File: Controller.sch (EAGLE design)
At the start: 5 parts

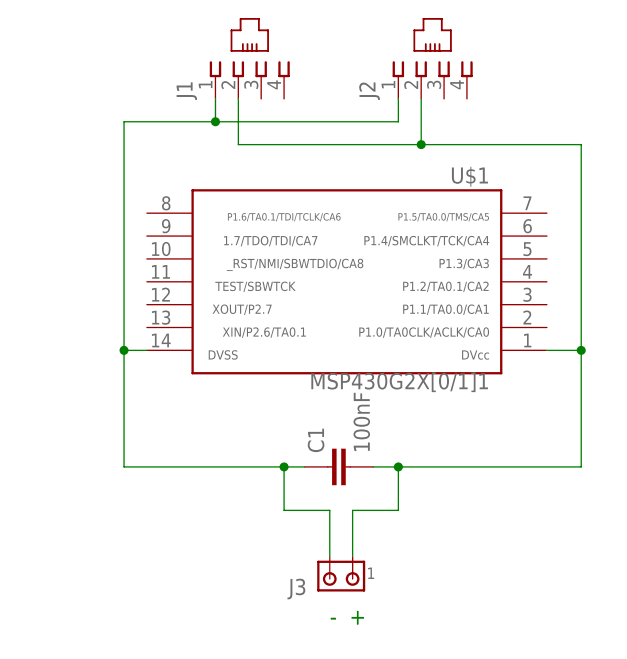
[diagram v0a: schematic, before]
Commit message: final schematics
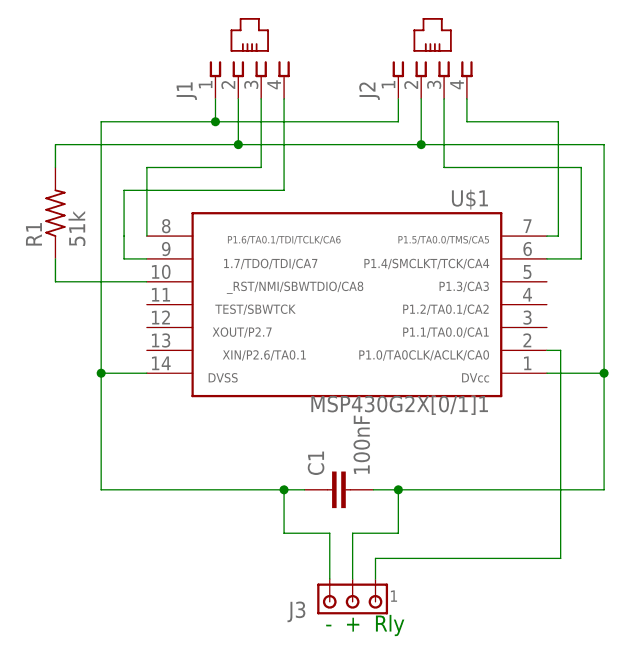
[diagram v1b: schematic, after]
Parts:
- added R1: 51k, resistor:R-US_R0603
- J3: device con-amp:MTA02-156 -> con-amp:MTA03-100
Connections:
- new net N$3: R1.1, U$1.10
- new net N$4: J1.3, U$1.8
- new net N$5: J1.4, U$1.9
- new net N$6: J3.1, U$1.2
- new net N$7: J2.4, U$1.7
- new net N$8: J2.3, U$1.6
- net N$1: now also J3.3; no longer J3.2
- net N$2: now also J3.2, R1.2; no longer J3.1
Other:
- note added: "- + Rly"
- note removed: "- +"
- moved on the sheet: C1, U$1
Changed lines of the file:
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@@
 <part name="J2" library="con-amp" deviceset="555166-3" device=""/>
 <part name="U$1" library="TI_MSP430_v16" deviceset="G2X[0/1]1---N14" device=""/>
-<part name="J3" library="con-amp" deviceset="MTA02-156" device=""/>
+<part name="J3" library="con-amp" deviceset="MTA03-100" device=""/>
 <part name="C1" library="capacitor-wima" deviceset="C" device="2.5/2" value="100nF"/>
+<part name="R1" library="resistor" deviceset="R-US_" device="R0603" value="51k"/>
 </parts>
 <sheets>
 <sheet>
 <plain>
-<text x="43.18" y="12.7" size="1.778" layer="91">-  +</text>
+<text x="42.672" y="11.938" size="1.778" layer="91">-  +  Rly</text>
 </plain>
 <instances>
 <instance part="J1" gate="G$1" x="35.56" y="73.66" rot="R90"/>
 <instance part="J2" gate="G$1" x="55.88" y="73.66" rot="R90"/>
-<instance part="U$1" gate="G$1" x="45.72" y="50.8" rot="R180"/>
-<instance part="J3" gate="G$1" x="45.72" y="17.78" rot="R180"/>
-<instance part="C1" gate="G$1" x="42.926" y="30.226" rot="R90"/>
+<instance part="U$1" gate="G$1" x="45.72" y="48.26" rot="R180"/>
+<instance part="J3" gate="G$1" x="45.72" y="15.24" rot="R180"/>
+<instance part="C1" gate="G$1" x="42.926" y="27.686" rot="R90"/>
+<instance part="R1" gate="G$1" x="12.7" y="58.42" rot="R90"/>
 </instances>
 <busses>
@@
 <segment>
 <pinref part="U$1" gate="G$1" pin="14"/>
-<wire x1="22.86" y1="43.18" x2="20.32" y2="43.18" width="0.1524" layer="91"/>
-<wire x1="20.32" y1="43.18" x2="20.32" y2="30.226" width="0.1524" layer="91"/>
-<wire x1="20.32" y1="30.226" x2="38.1" y2="30.226" width="0.1524" layer="91"/>
-<wire x1="40.386" y1="30.226" x2="38.1" y2="30.226" width="0.1524" layer="91"/>
-<wire x1="38.1" y1="30.226" x2="38.1" y2="25.4" width="0.1524" layer="91"/>
-<pinref part="J3" gate="G$1" pin="2"/>
-<wire x1="38.1" y1="25.4" x2="43.18" y2="25.4" width="0.1524" layer="91"/>
-<wire x1="43.18" y1="25.4" x2="43.18" y2="20.32" width="0.1524" layer="91"/>
-<junction x="38.1" y="30.226"/>
-<wire x1="20.32" y1="43.18" x2="20.32" y2="68.58" width="0.1524" layer="91"/>
+<wire x1="22.86" y1="40.64" x2="17.78" y2="40.64" width="0.1524" layer="91"/>
+<wire x1="17.78" y1="40.64" x2="17.78" y2="27.686" width="0.1524" layer="91"/>
+<wire x1="17.78" y1="27.686" x2="38.1" y2="27.686" width="0.1524" layer="91"/>
+<wire x1="40.386" y1="27.686" x2="38.1" y2="27.686" width="0.1524" layer="91"/>
+<wire x1="38.1" y1="27.686" x2="38.1" y2="22.86" width="0.1524" layer="91"/>
+<pinref part="J3" gate="G$1" pin="3"/>
+<wire x1="38.1" y1="22.86" x2="43.18" y2="22.86" width="0.1524" layer="91"/>
+<wire x1="43.18" y1="22.86" x2="43.18" y2="17.78" width="0.1524" layer="91"/>
+<junction x="38.1" y="27.686"/>
+<wire x1="17.78" y1="40.64" x2="17.78" y2="68.58" width="0.1524" layer="91"/>
 <pinref part="J2" gate="G$1" pin="1"/>
 <wire x1="50.8" y1="71.12" x2="50.8" y2="68.58" width="0.1524" layer="91"/>
@@
 <wire x1="50.8" y1="68.58" x2="30.48" y2="68.58" width="0.1524" layer="91"/>
 <wire x1="30.48" y1="68.58" x2="30.48" y2="71.12" width="0.1524" layer="91"/>
-<wire x1="20.32" y1="68.58" x2="30.48" y2="68.58" width="0.1524" layer="91"/>
+<wire x1="17.78" y1="68.58" x2="30.48" y2="68.58" width="0.1524" layer="91"/>
 <junction x="30.48" y="68.58"/>
-<junction x="20.32" y="43.18"/>
+<junction x="17.78" y="40.64"/>
 <pinref part="C1" gate="G$1" pin="1"/>
 </segment>
@@
 <net name="N$2" class="0">
 <segment>
-<pinref part="J3" gate="G$1" pin="1"/>
-<wire x1="45.72" y1="20.32" x2="45.72" y2="25.4" width="0.1524" layer="91"/>
-<wire x1="45.72" y1="25.4" x2="50.8" y2="25.4" width="0.1524" layer="91"/>
-<wire x1="50.8" y1="25.4" x2="50.8" y2="30.226" width="0.1524" layer="91"/>
-<wire x1="50.8" y1="30.226" x2="48.006" y2="30.226" width="0.1524" layer="91"/>
-<wire x1="50.8" y1="30.226" x2="71.12" y2="30.226" width="0.1524" layer="91"/>
-<junction x="50.8" y="30.226"/>
+<pinref part="J3" gate="G$1" pin="2"/>
+<wire x1="45.72" y1="17.78" x2="45.72" y2="22.86" width="0.1524" layer="91"/>
+<wire x1="45.72" y1="22.86" x2="50.8" y2="22.86" width="0.1524" layer="91"/>
+<wire x1="50.8" y1="22.86" x2="50.8" y2="27.686" width="0.1524" layer="91"/>
+<wire x1="50.8" y1="27.686" x2="48.006" y2="27.686" width="0.1524" layer="91"/>
+<wire x1="50.8" y1="27.686" x2="73.66" y2="27.686" width="0.1524" layer="91"/>
+<junction x="50.8" y="27.686"/>
 <pinref part="J2" gate="G$1" pin="2"/>
 <wire x1="53.34" y1="71.12" x2="53.34" y2="66.04" width="0.1524" layer="91"/>
@@
 <wire x1="53.34" y1="66.04" x2="33.02" y2="66.04" width="0.1524" layer="91"/>
 <wire x1="33.02" y1="66.04" x2="33.02" y2="71.12" width="0.1524" layer="91"/>
-<wire x1="53.34" y1="66.04" x2="71.12" y2="66.04" width="0.1524" layer="91"/>
-<wire x1="71.12" y1="66.04" x2="71.12" y2="43.18" width="0.1524" layer="91"/>
+<wire x1="53.34" y1="66.04" x2="73.66" y2="66.04" width="0.1524" layer="91"/>
 <junction x="53.34" y="66.04"/>
-<wire x1="71.12" y1="43.18" x2="71.12" y2="30.226" width="0.1524" layer="91"/>
-<wire x1="67.31" y1="43.18" x2="71.12" y2="43.18" width="0.1524" layer="91"/>
+<wire x1="73.66" y1="40.64" x2="73.66" y2="27.686" width="0.1524" layer="91"/>
+<wire x1="67.31" y1="40.64" x2="73.66" y2="40.64" width="0.1524" layer="91"/>
 <pinref part="U$1" gate="G$1" pin="1"/>
-<junction x="71.12" y="43.18"/>
+<junction x="73.66" y="40.64"/>
 <pinref part="C1" gate="G$1" pin="2"/>
+<pinref part="R1" gate="G$1" pin="2"/>
+<wire x1="12.7" y1="63.5" x2="12.7" y2="66.04" width="0.1524" layer="91"/>
+<wire x1="12.7" y1="66.04" x2="33.02" y2="66.04" width="0.1524" layer="91"/>
+<junction x="33.02" y="66.04"/>
+<wire x1="73.66" y1="66.04" x2="73.66" y2="40.64" width="0.1524" layer="91"/>
 </segment>
 </net>
+<net name="N$3" class="0">
+<segment>
+<pinref part="U$1" gate="G$1" pin="10"/>
+<pinref part="R1" gate="G$1" pin="1"/>
+<wire x1="22.86" y1="50.8" x2="12.7" y2="50.8" width="0.1524" layer="91"/>
+<wire x1="12.7" y1="50.8" x2="12.7" y2="53.34" width="0.1524" layer="91"/>
+</segment>
+</net>
+<net name="N$4" class="0">
+<segment>
+<pinref part="J1" gate="G$1" pin="3"/>
+<wire x1="35.56" y1="71.12" x2="35.56" y2="63.5" width="0.1524" layer="91"/>
+<pinref part="U$1" gate="G$1" pin="8"/>
+<wire x1="35.56" y1="63.5" x2="22.86" y2="63.5" width="0.1524" layer="91"/>
+<wire x1="22.86" y1="63.5" x2="22.86" y2="55.88" width="0.1524" layer="91"/>
+</segment>
+</net>
+<net name="N$5" class="0">
+<segment>
+<pinref part="U$1" gate="G$1" pin="9"/>
+<pinref part="J1" gate="G$1" pin="4"/>
+<wire x1="22.86" y1="53.34" x2="20.32" y2="53.34" width="0.1524" layer="91"/>
+<wire x1="20.32" y1="53.34" x2="20.32" y2="55.88" width="0.1524" layer="91"/>
+<wire x1="20.32" y1="55.88" x2="20.32" y2="60.96" width="0.1524" layer="91"/>
+<wire x1="20.32" y1="60.96" x2="38.1" y2="60.96" width="0.1524" layer="91"/>
+<wire x1="38.1" y1="60.96" x2="38.1" y2="71.12" width="0.1524" layer="91"/>
+</segment>
+</net>
+<net name="N$7" class="0">
+<segment>
+<pinref part="J2" gate="G$1" pin="4"/>
+<wire x1="68.58" y1="68.58" x2="58.42" y2="68.58" width="0.1524" layer="91"/>
+<wire x1="58.42" y1="68.58" x2="58.42" y2="71.12" width="0.1524" layer="91"/>
+<wire x1="68.58" y1="68.58" x2="68.58" y2="55.88" width="0.1524" layer="91"/>
+<pinref part="U$1" gate="G$1" pin="7"/>
+<wire x1="68.58" y1="55.88" x2="67.31" y2="55.88" width="0.1524" layer="91"/>
+</segment>
+</net>
+<net name="N$8" class="0">
+<segment>
+<pinref part="J2" gate="G$1" pin="3"/>
+<wire x1="55.88" y1="71.12" x2="55.88" y2="63.5" width="0.1524" layer="91"/>
+<wire x1="55.88" y1="63.5" x2="71.12" y2="63.5" width="0.1524" layer="91"/>
+<wire x1="71.12" y1="63.5" x2="71.12" y2="53.34" width="0.1524" layer="91"/>
+<pinref part="U$1" gate="G$1" pin="6"/>
+<wire x1="71.12" y1="53.34" x2="67.31" y2="53.34" width="0.1524" layer="91"/>
+</segment>
+</net>
+<net name="N$6" class="0">
+<segment>
+<pinref part="U$1" gate="G$1" pin="2"/>
+<wire x1="67.31" y1="43.18" x2="68.834" y2="43.18" width="0.1524" layer="91"/>
+<wire x1="68.834" y1="43.18" x2="68.834" y2="20.066" width="0.1524" layer="91"/>
+<pinref part="J3" gate="G$1" pin="1"/>
+<wire x1="68.834" y1="20.066" x2="48.26" y2="20.066" width="0.1524" layer="91"/>
+<wire x1="48.26" y1="20.066" x2="48.26" y2="17.78" width="0.1524" layer="91"/>
+</segment>
+</net>
